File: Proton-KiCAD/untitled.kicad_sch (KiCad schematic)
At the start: 45 parts, among them J11 FRONT_BUTTON_1, J12 FRONT_BUTTON_2, J2 KEYPAD, J3 SJ-43514, J4 SPEAKER_OUT, J5 OLED SPI, J6 ROTARY ENCODER, J7 OLED, J8 SI4703, U5 TL072, U6 LM386

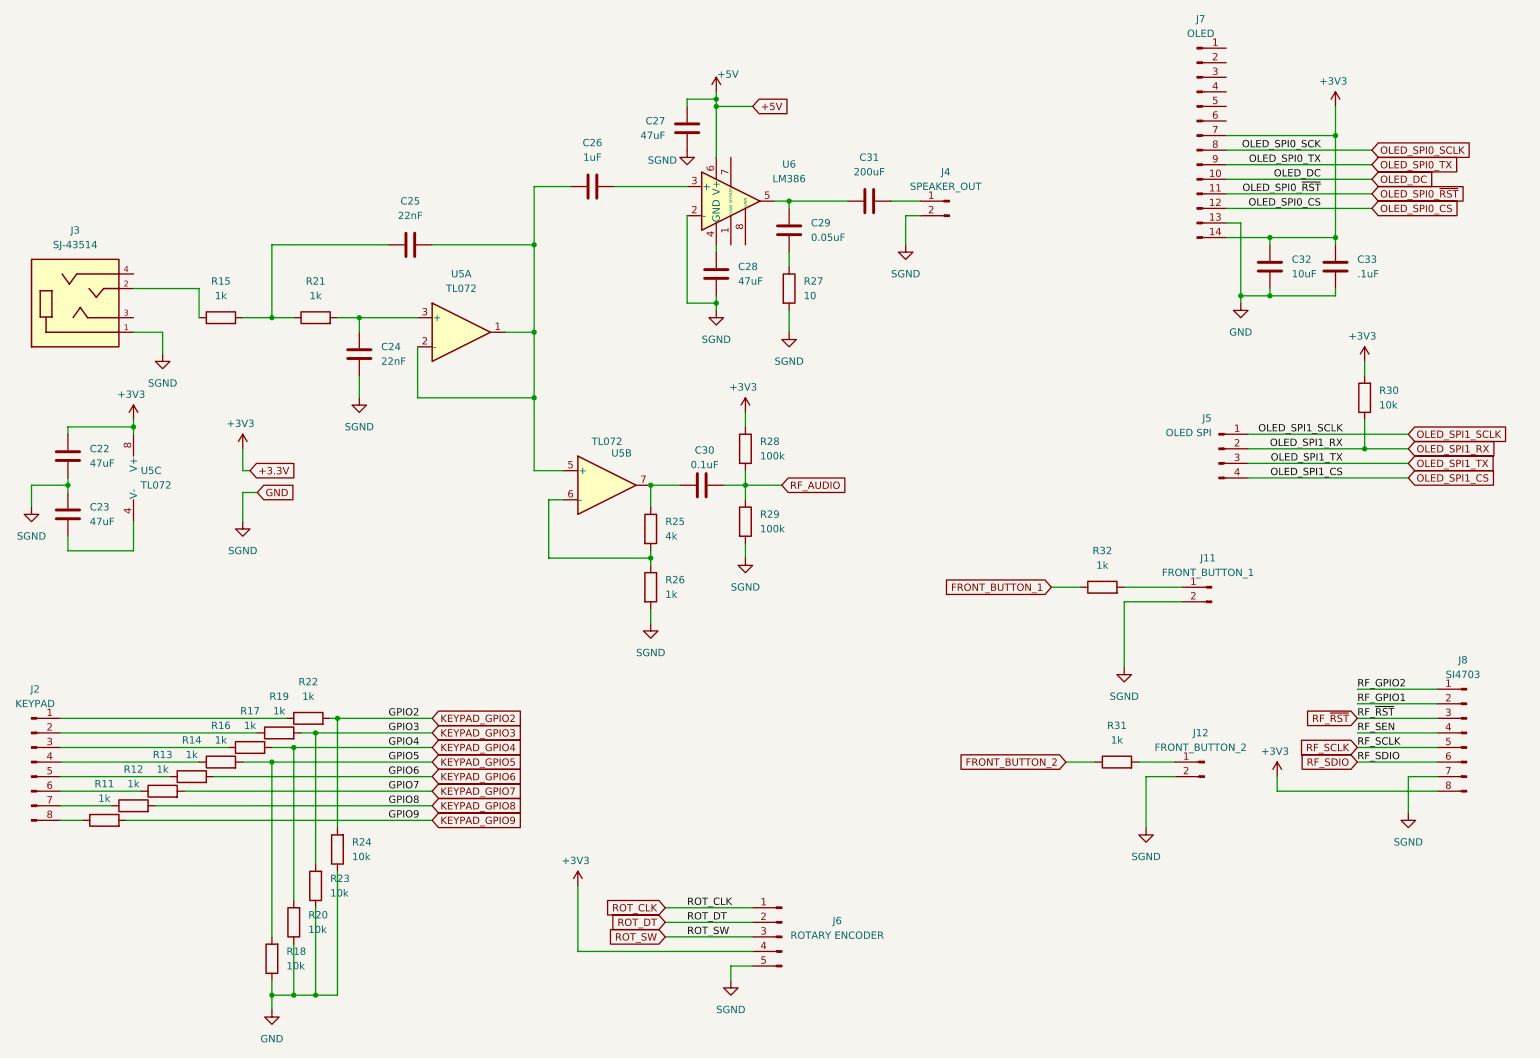
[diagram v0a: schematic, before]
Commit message: fixed audio section
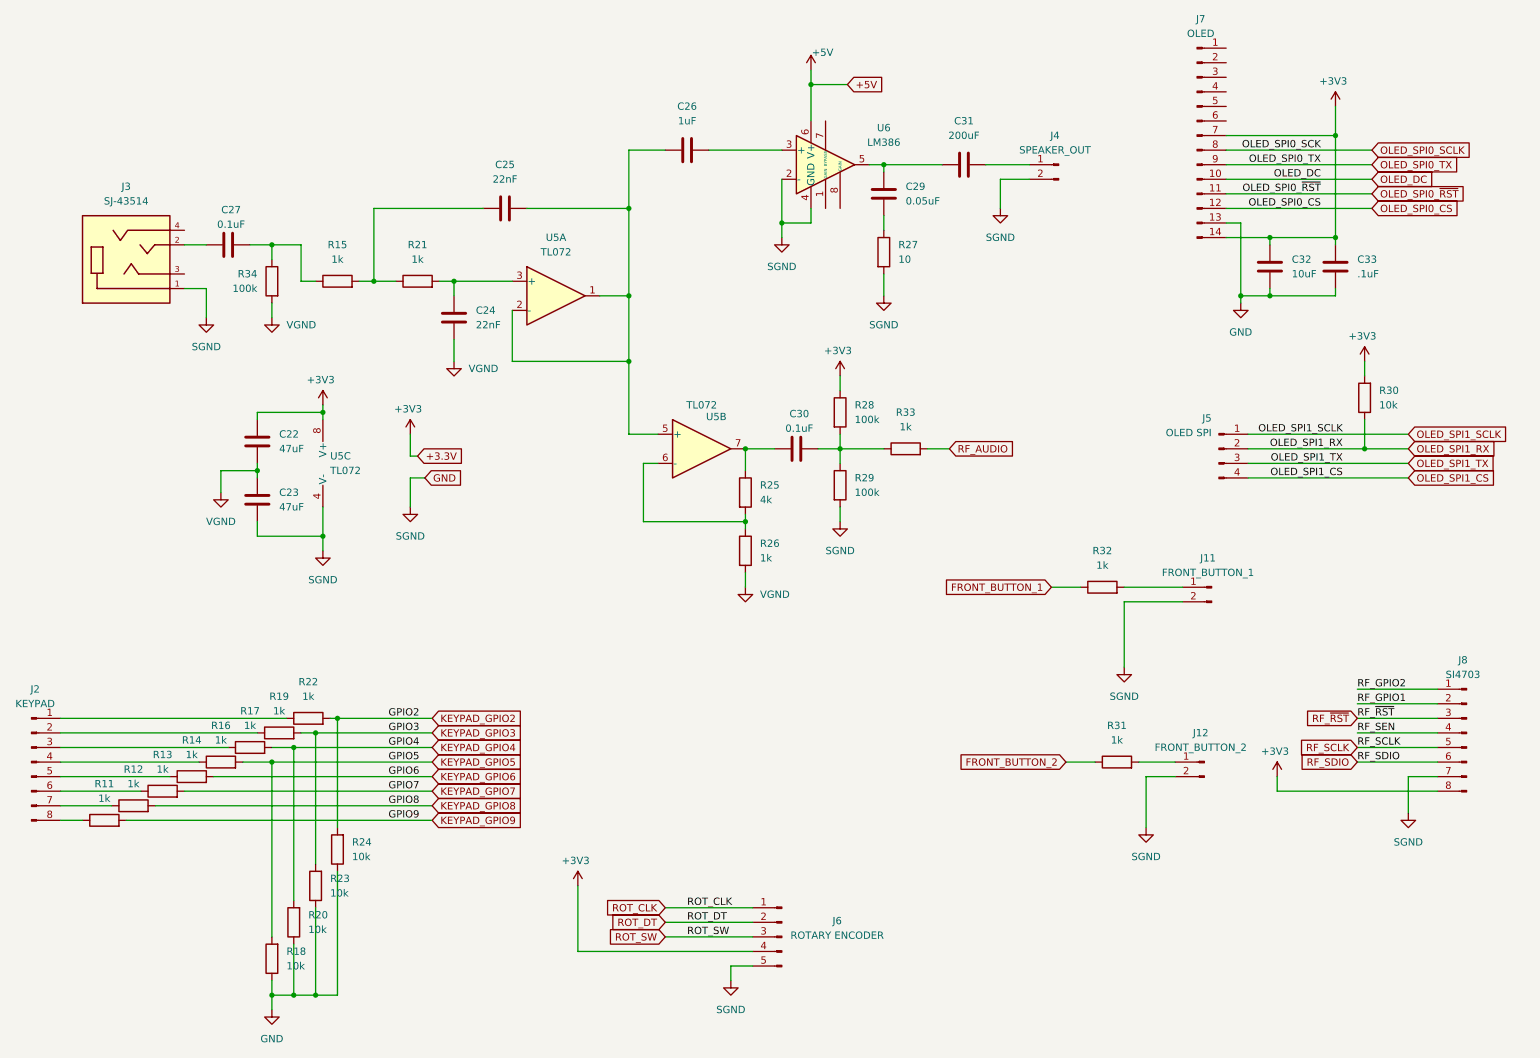
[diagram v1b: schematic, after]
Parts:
- removed C28: 47uF, Capacitor_SMD:C_0805_2012Metric, symbol Device:C
- added R33: 1k, Resistor_SMD:R_0402_1005Metric, symbol Device:R
- added R34: 100k, Resistor_SMD:R_0402_1005Metric, symbol Device:R
- C27: value 47uF -> 0.1uF; footprint Capacitor_SMD:C_0805_2012Metric -> Capacitor_SMD:C_0402_1005Metric
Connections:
- net +5V: no longer C27.1
- net GND: now also C23.2, U5.4 (V-), U6.4 (GND); no longer C22.2, C23.1, C24.2, C27.2, R26.2
- net RF_AUDIO: now also R33.2; no longer C30.2, R28.2, R29.1
- net at R15.1: now also C27.2, R34.1; no longer J3.2
- new net: C30.2, R28.2, R29.1, R33.1
- new net: C27.1, J3.2
- new net VGND: C22.2, C23.1, C24.2, R26.2, R34.2
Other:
- moved on the sheet: C22, C23, C24, C25, C26, C29, C30, C31, J3, J4, R15, R21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
